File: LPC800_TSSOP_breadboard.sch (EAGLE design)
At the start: 17 parts, among them Q1 12MHz

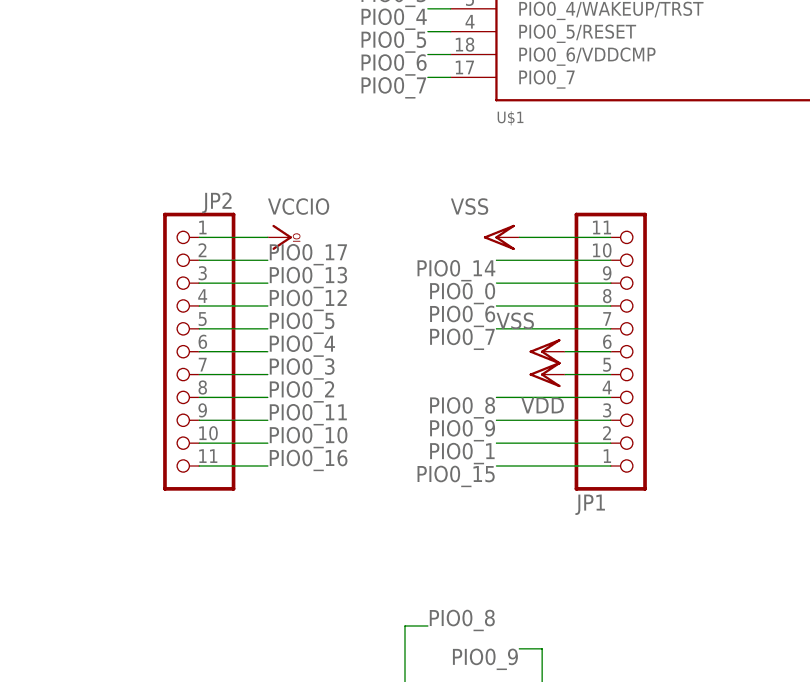
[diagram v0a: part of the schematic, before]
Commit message: * updated board and schem with todo's
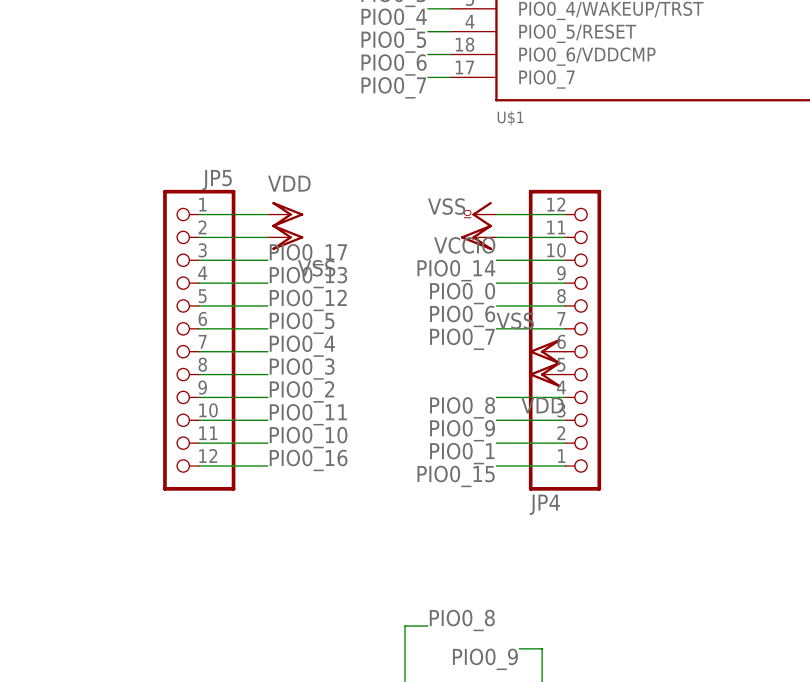
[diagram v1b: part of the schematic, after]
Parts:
- removed JP1, JP2: (no value), bart_connectors:PINHD-1X11TH_SMALL
- added JP4, JP5: (no value), SquantorConnectors:PINHD-1X12SMALL
- C4, C5: device bart_rcl:C-EUC0805 -> bart_rcl:C-EUC0805K
- renumbered LOGO1 to LOGO2
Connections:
- net PIO0_0: now also JP4.9; no longer JP1.9
- net PIO0_1: now also JP4.2; no longer JP1.2
- net PIO0_10: now also JP5.11; no longer JP2.10
- net PIO0_11: now also JP5.10; no longer JP2.9
- net PIO0_12: now also JP5.5; no longer JP2.4
- net PIO0_13: now also JP5.4; no longer JP2.3
- net PIO0_14: now also JP4.10; no longer JP1.10
- net PIO0_15: now also JP4.1; no longer JP1.1
- net PIO0_16: now also JP5.12; no longer JP2.11
- net PIO0_17: now also JP5.3; no longer JP2.2
- net PIO0_2: now also JP5.9; no longer JP2.8
- net PIO0_3: now also JP5.8; no longer JP2.7
- net PIO0_4: now also JP5.7; no longer JP2.6
- net PIO0_5: now also JP5.6; no longer JP2.5
- net PIO0_6: now also JP4.8; no longer JP1.8
- net PIO0_7: now also JP4.7; no longer JP1.7
- net PIO0_8: now also JP4.4; no longer JP1.4
- net PIO0_9: now also JP4.3; no longer JP1.3
- net VCCIO: now also JP4.12; no longer JP2.1
- net VDD: now also JP4.5, JP5.1; no longer JP1.5
- net VSS: now also JP4.11, JP4.6, JP5.2; no longer JP1.11, JP1.6
